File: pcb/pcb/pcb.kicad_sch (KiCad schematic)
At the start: 16 parts, among them J1 Conn_01x28_Socket, J2 Conn_01x28_Socket, J3 Conn_01x03_Socket, J4 Conn_01x04_Socket, J5 MAX17048, J6 LSM6DS3TR-C, J7 SSD1306

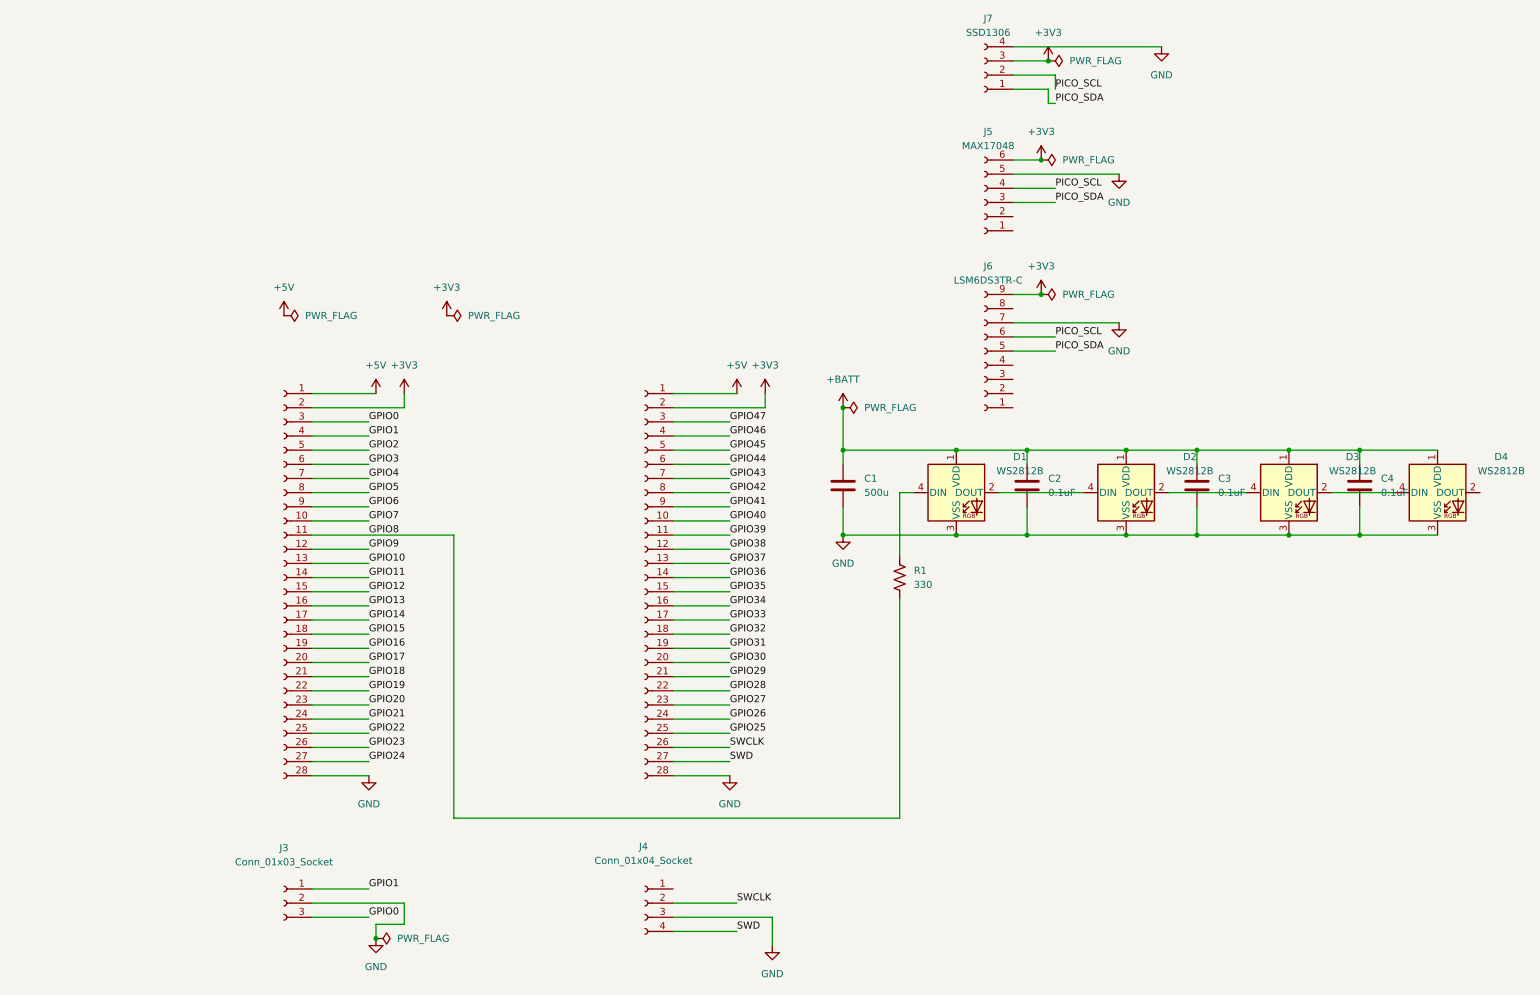
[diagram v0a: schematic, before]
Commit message: hopefully done w/ schmematic
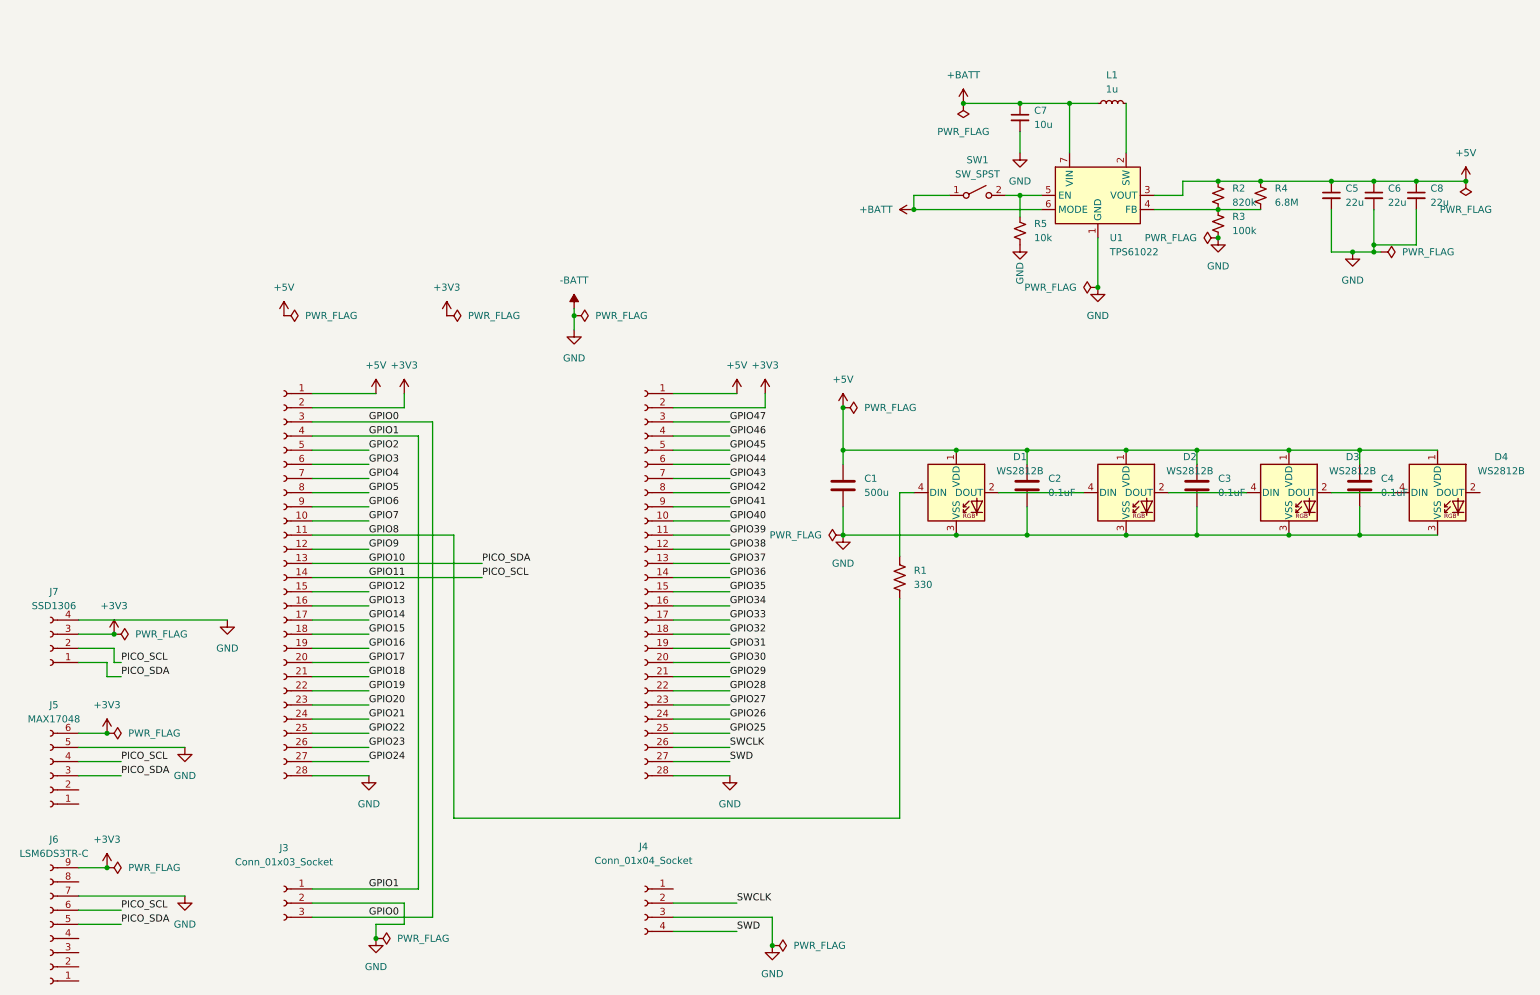
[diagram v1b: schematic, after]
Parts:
- added C5, C6, C8: 22u, symbol Device:C_Small
- added C7: 10u, symbol Device:C_Small
- added L1: 1u, symbol Device:L_Small
- added R2: 820k, symbol Device:R_Small_US
- added R3: 100k, symbol Device:R_Small_US
- added R4: 6.8M, symbol Device:R_Small_US
- added R5: 10k, symbol Device:R_Small_US
- added SW1: SW_SPST, symbol Switch:SW_SPST
- added U1: TPS61022, Package_DFN_QFN:Texas_RWU0007A_VQFN-7_2x2mm_P0.5mm, symbol Converter_DCDC:TPS61022
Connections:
- net PICO_SCL is gone; now on net GPIO11: J5.4 (Pin_4), J6.6 (Pin_6), J7.2 (Pin_2)
- net PICO_SDA is gone; now on net GPIO10: J5.3 (Pin_3), J6.5 (Pin_5), J7.1 (Pin_1)
- net +5V: now also C1.1, C2.1, C3.1, C4.1, D1.1 (VDD), D2.1 (VDD), D3.1 (VDD), D4.1 (VDD), C5.1, C6.1, C8.1, R2.1, R4.1, U1.3 (VOUT)
- net +BATT: now also C7.1, L1.1, SW1.1 (A), U1.6 (MODE), U1.7 (VIN); no longer C1.1, C2.1, C3.1, C4.1, D1.1 (VDD), D2.1 (VDD), D3.1 (VDD), D4.1 (VDD)
- net GND renamed -BATT
- net -BATT: now also C5.2, C6.2, C7.2, C8.2, R3.2, R5.2, U1.1 (GND)
- new net: R5.1, SW1.2 (B), U1.5 (EN)
- new net: R2.2, R3.1, R4.2, U1.4 (FB)
- new net: L1.2, U1.2 (SW)
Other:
- moved on the sheet: J5, J6, J7
